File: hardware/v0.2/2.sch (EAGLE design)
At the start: 26 parts, among them IC2 STM32F10XCXT6, U1 ADXL345"

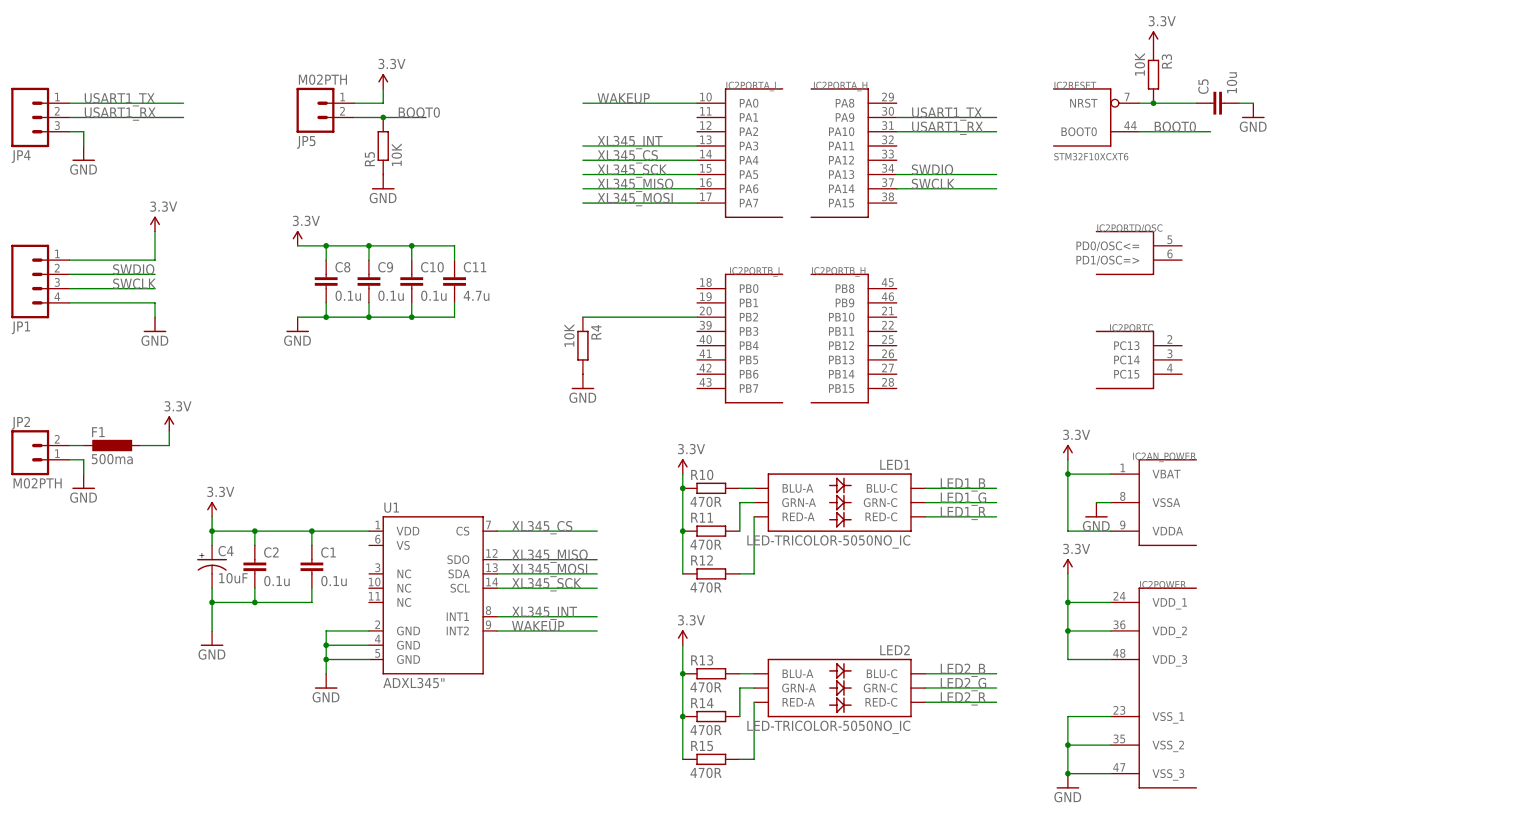
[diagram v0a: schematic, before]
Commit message: modify pcb design
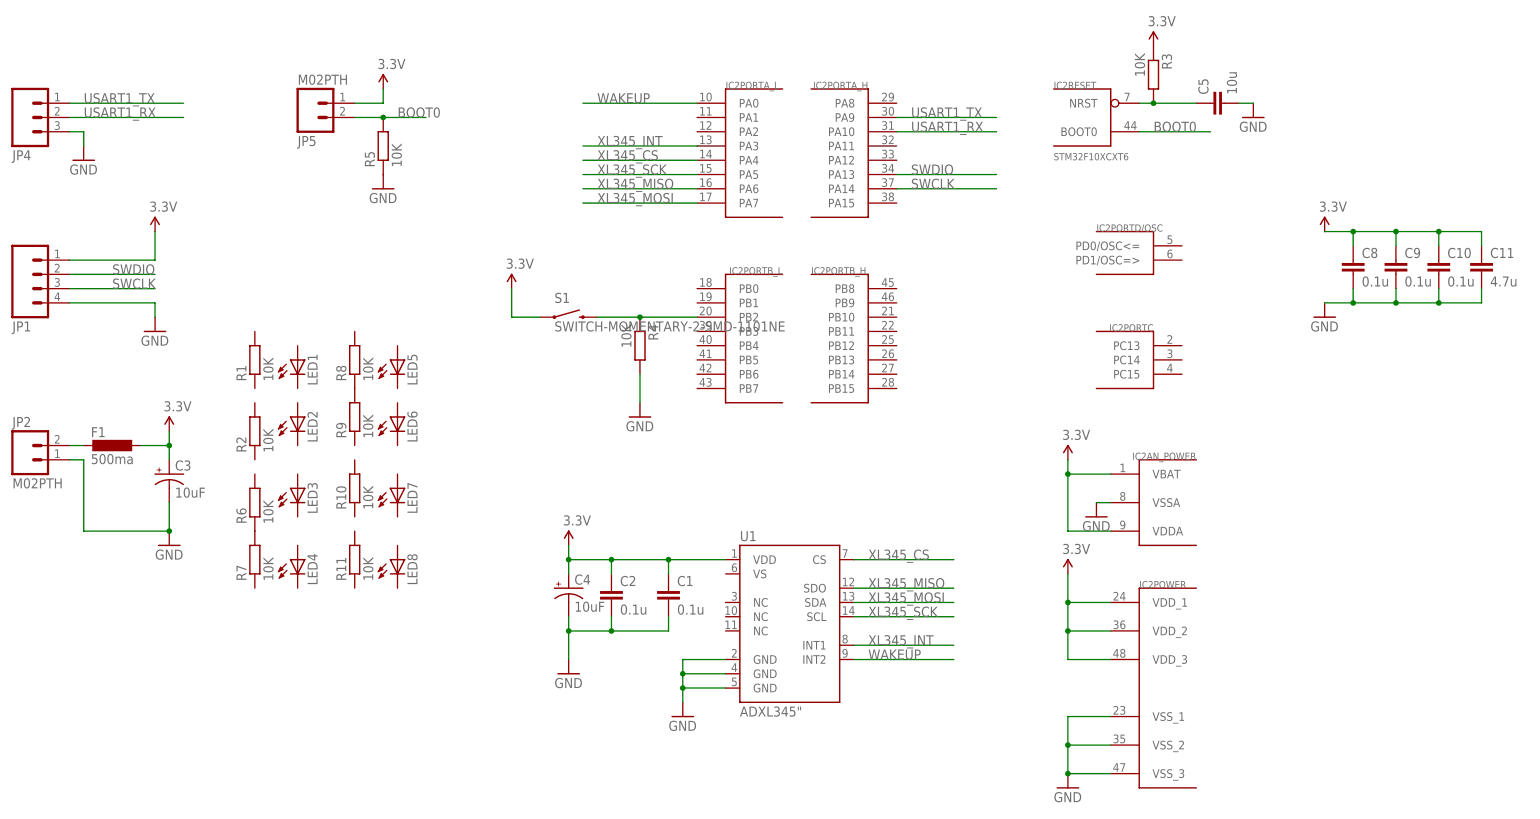
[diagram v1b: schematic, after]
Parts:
- removed R12, R13, R14, R15: 470R, rcl:R-EU_R0603
- added C3: 10uF, SparkFun-Capacitors:10UF-16V-10%(TANT)
- added LED3, LED4, LED5, LED6, LED7, LED8: (no value), SparkFun-LED:LED1206
- added R1, R2, R6, R7, R8, R9: 10K, rcl:R-EU_R0603
- added S1: SWITCH-MOMENTARY-2-SMD-1101NE, SparkFun-Electromechanical:SWITCH-MOMENTARY-2-SMD-1101NE
- LED1, LED2: value LED-TRICOLOR-5050NO_IC -> (none); device SparkFun-LED:LED-TRICOLOR-5050NO_IC -> SparkFun-LED:LED1206
- R10, R11: value 470R -> 10K
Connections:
- removed net LED1_B: LED1.BLU-C
- removed net LED1_G: LED1.GRN-C
- removed net LED1_R: LED1.RED-C
- removed net LED2_B: LED2.BLU-C
- removed net LED2_G: LED2.GRN-C
- removed net LED2_R: LED2.RED-C
- removed net N$10: LED1.GRN-A, R11.2
- removed net N$11: LED1.RED-A, R12.2
- removed net N$12: LED2.BLU-A, R13.2
- removed net N$13: LED2.GRN-A, R14.2
- removed net N$14: LED2.RED-A, R15.2
- removed net N$8: LED1.BLU-A, R10.2
- new net N$3: R6.1, R7.2
- new net N$4: R8.1, R9.2
- net 3.3V: now also C3.+, S1.1; no longer R10.1, R11.1, R12.1, R13.1, R14.1, R15.1
- net GND: now also C3.-
- net N$2: now also S1.2
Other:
- moved on the sheet: C1, C10, C11, C2, C4, C8, C9, R10, R11, R4, U1
